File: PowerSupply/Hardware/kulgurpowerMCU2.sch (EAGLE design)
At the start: 143 parts, among them IC2 TPS77333DGK, IC3 REG1117-5, U1 MPU-6000QFN-24, U2 MPU-6000QFN-24, X1 12Mhz, X2 2534-, X3 22-23-2021

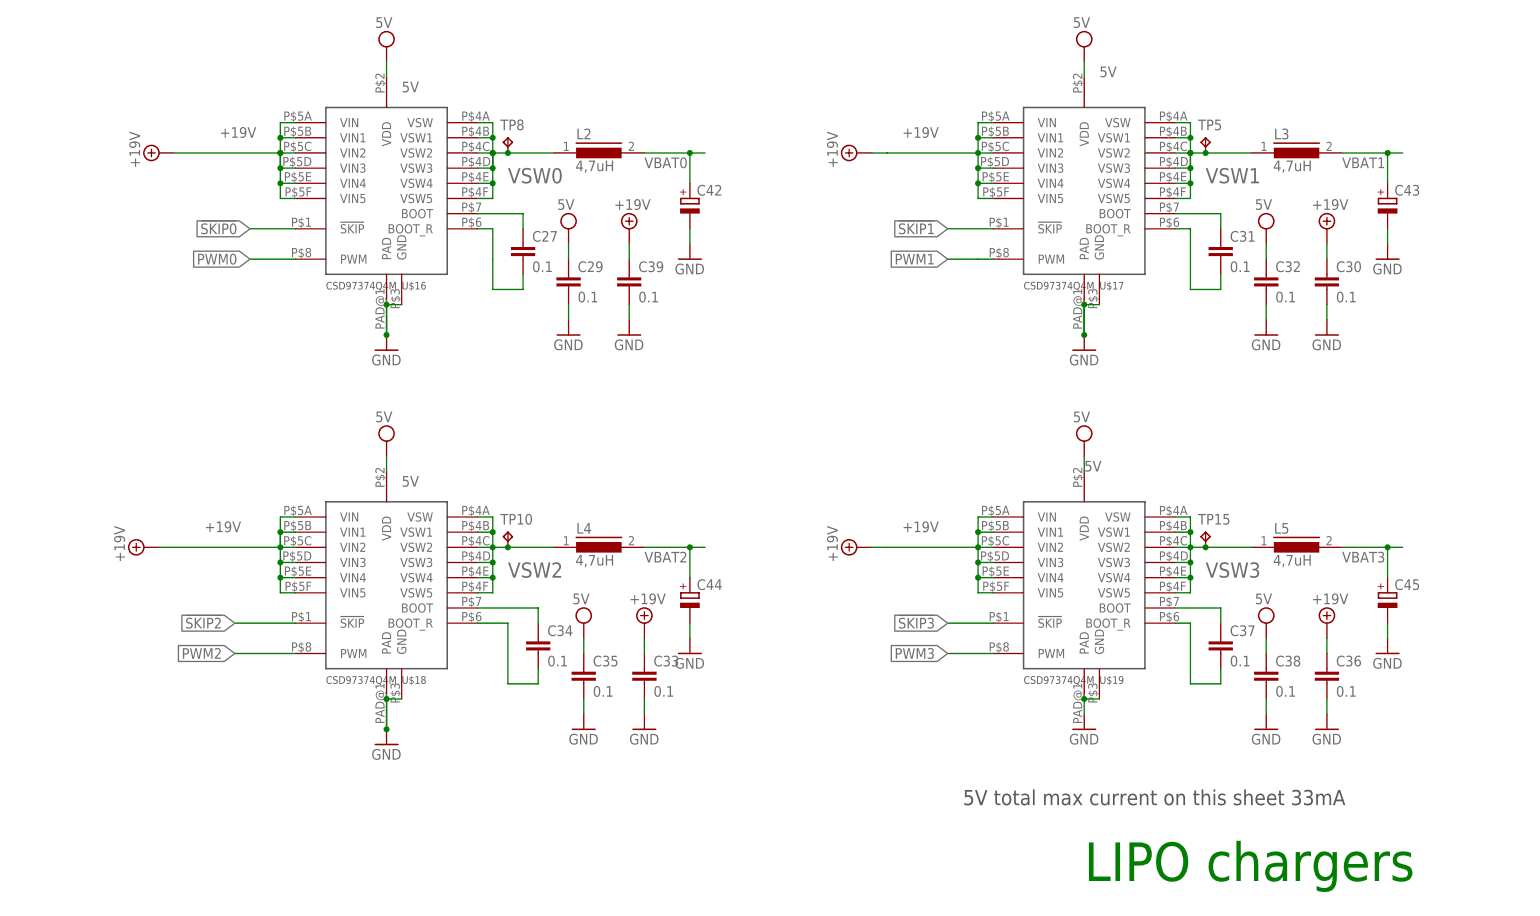
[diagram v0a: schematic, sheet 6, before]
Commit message: Minor bugfixes to boards.
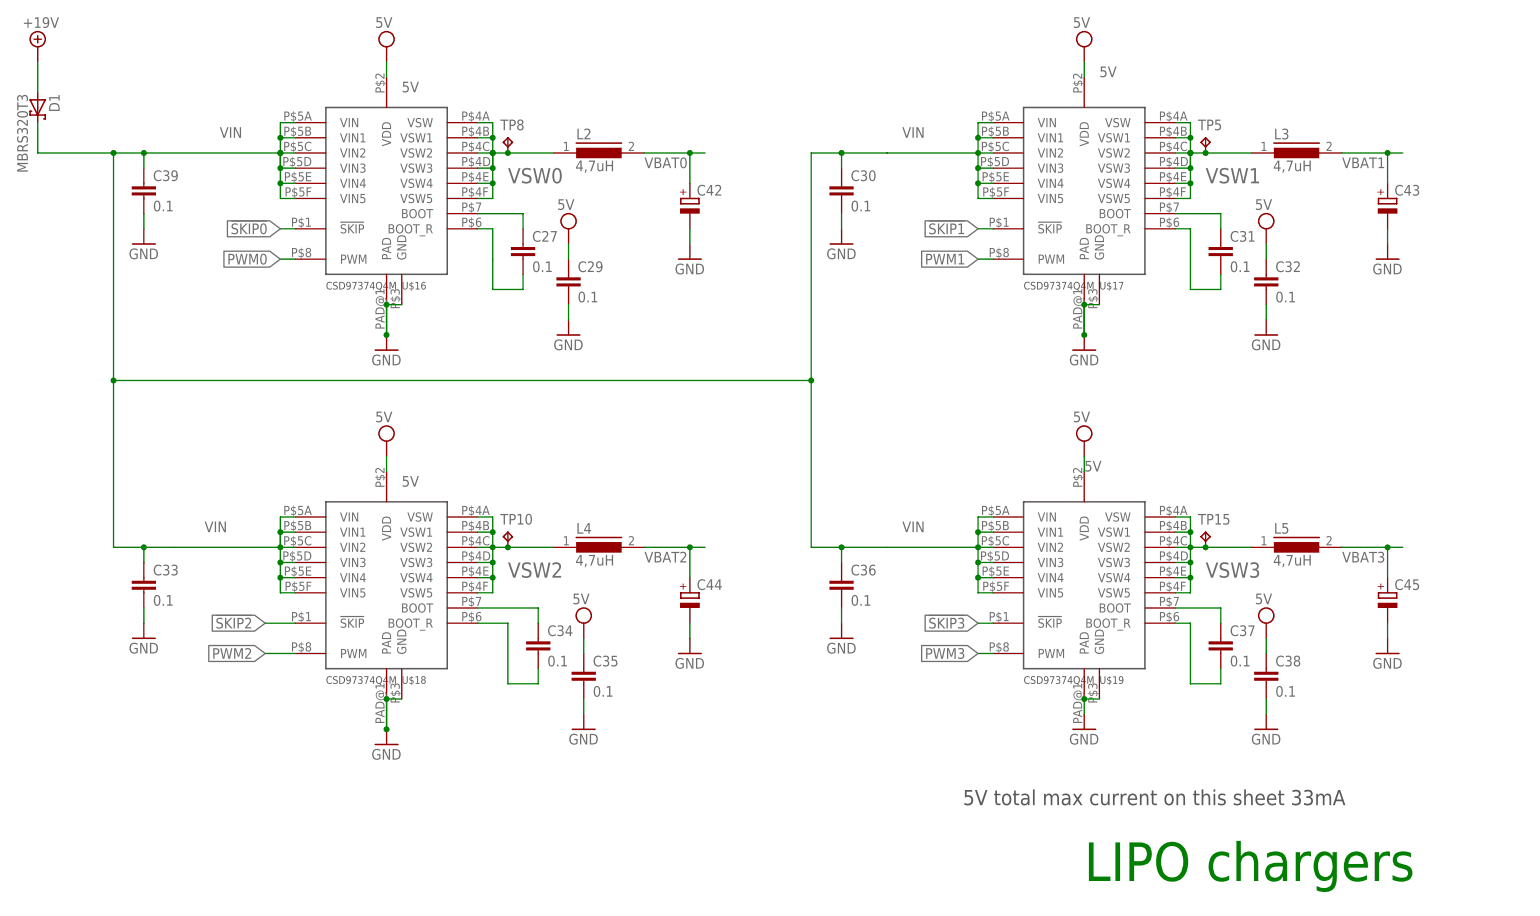
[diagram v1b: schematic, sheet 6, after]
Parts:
- added D1: MBRS320T3, diode:MBRS320T3
- D8: value LED-RGB-CC-THRUDIFFUSE -> WP154A4SUREQBFZGW
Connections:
- net EN_PANDA1 renamed BUZZER_X
- new net VIN: C30.1, C33.1, C36.1, C39.1, D1.C, U$16.VIN, U$16.VIN1, U$16.VIN2, U$16.VIN3, U$16.VIN4, U$16.VIN5, U$17.VIN, U$17.VIN1, U$17.VIN2, U$17.VIN3, U$17.VIN4, U$17.VIN5, U$18.VIN, U$18.VIN1, U$18.VIN2, U$18.VIN3, U$18.VIN4, U$18.VIN5, U$19.VIN, U$19.VIN1, U$19.VIN2, U$19.VIN3, U$19.VIN4, U$19.VIN5
- net +19V: now also D1.A; no longer C30.1, C33.1, C36.1, C39.1, U$16.VIN, U$16.VIN1, U$16.VIN2, U$16.VIN3, U$16.VIN4, U$16.VIN5, U$17.VIN, U$17.VIN1, U$17.VIN2, U$17.VIN3, U$17.VIN4, U$17.VIN5, U$18.VIN, U$18.VIN1, U$18.VIN2, U$18.VIN3, U$18.VIN4, U$18.VIN5, U$19.VIN, U$19.VIN1, U$19.VIN2, U$19.VIN3, U$19.VIN4, U$19.VIN5
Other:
- moved on the sheet: C30, C33, C36, C39, U2
